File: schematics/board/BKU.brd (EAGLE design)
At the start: 94 x 94 mm, 73 parts, among them Q1 8MHz, Q2 32,768KHz, U1 STM32F405RGT6

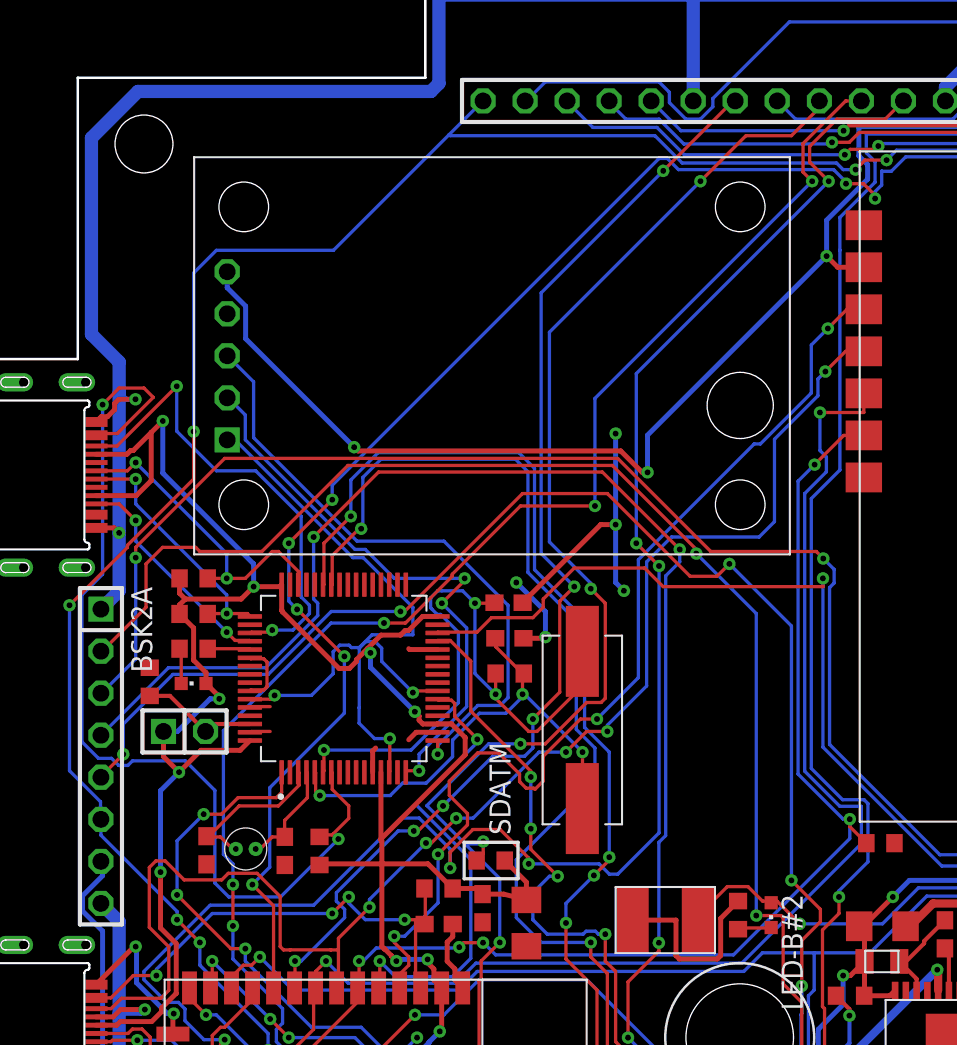
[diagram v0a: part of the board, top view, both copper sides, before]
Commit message: Изменения в подключении мк
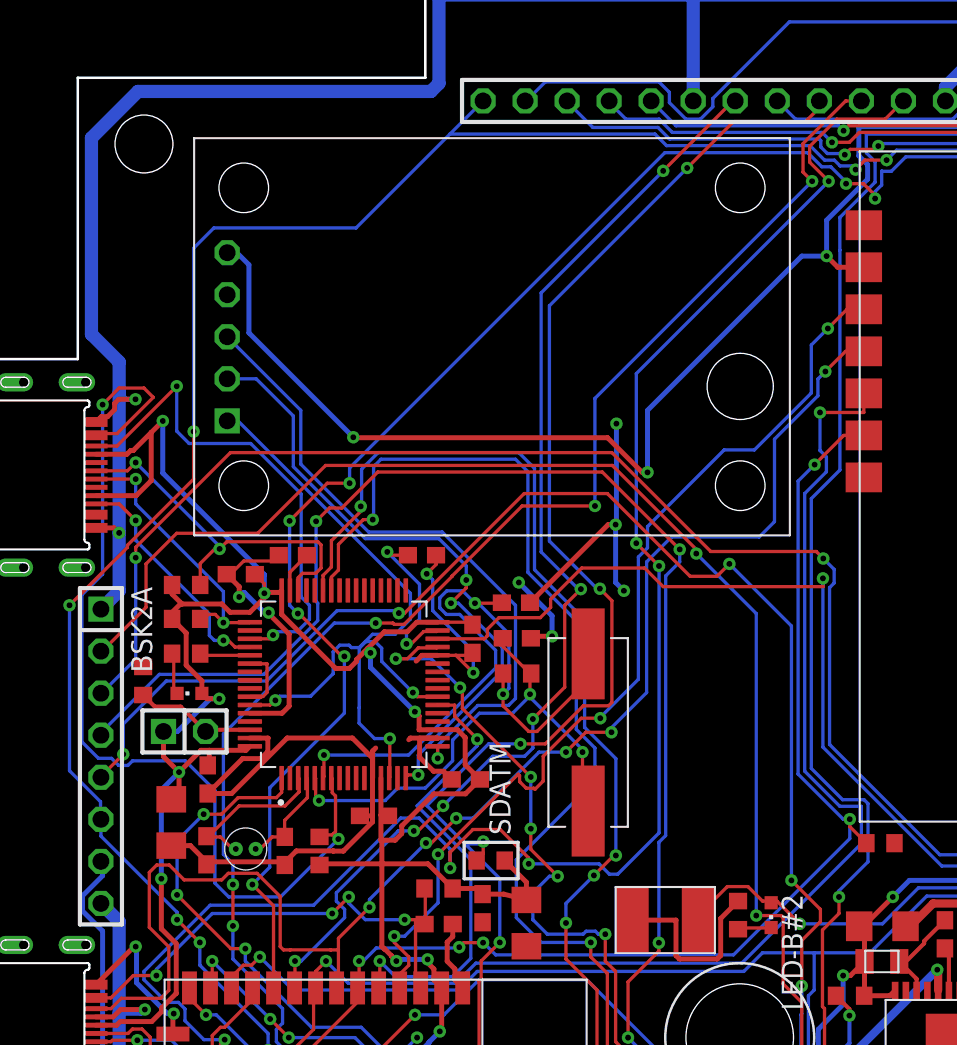
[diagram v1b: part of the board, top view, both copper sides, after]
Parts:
- added C13, C9: 2,2µ, rcl:C0603
- added C18, C20, C53, C54, C55: 100nF, rcl:C0603
- added C19: 10µ, rcl:C1206
- moved GPS 1.15 mm to (31.0, 72.3)
- moved LED2 0.65 mm to (12.8, 50.8)
- moved R1 0.60 mm to (12.6, 57.4)
- moved R3 0.54 mm to (12.6, 55.3)
- moved R15 0.54 mm to (12.6, 53.2)
- moved C7 0.45 mm to (32.5, 54.1)
- moved C8 0.45 mm to (32.5, 56.3)
- moved R17 0.45 mm to (32.5, 52.0)
- moved R14 0.40 mm to (9.95, 51.5)
- moved Q1 0.38 mm to (36.8, 48.4)
- moved U1 0.35 mm to (22.1, 51.4)
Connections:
- removed net VCAP_1: U1.31
- removed net VCAP_2: U1.47
- new net N$7: C9.2, U1.31
- new net N$8: C13.2, U1.47
- net GND: now also C13.1, C18.1, C19.1, C20.1, C53.1, C54.1, C55.1, C9.1
- net VDD: now also C18.2, C19.2, C20.2, C53.2, C54.2, C55.2
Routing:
- net GND: track 460.7 -> 530.7 mm, vias 24 -> 28
- net VDD: track 456.1 -> 466.6 mm
- net N$7: track 0.00 -> 10.2 mm, vias 0 -> 2
- net N$41: track 34.6 -> 38.5 mm
- net SWD: track 19.4 -> 23.0 mm
- net SCL: track 87.6 -> 91.1 mm, vias 8 -> 10
- net AUX: track 61.5 -> 58.2 mm
- net N$15: track 39.0 -> 41.6 mm
- net N$8: track 0.00 -> 2.56 mm
- net 5V: track 297.3 -> 299.4 mm
- net SDATM: track 108.4 -> 110.2 mm
- net SWC: track 15.4 -> 17.2 mm
- net N$42: track 37.6 -> 39.1 mm
- net RX-S: track 28.9 -> 30.2 mm
- net DS: track 122.2 -> 123.4 mm
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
